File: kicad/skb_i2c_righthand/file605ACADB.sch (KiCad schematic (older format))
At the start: 108 parts, among them SW1 SW_PUSH, SW10 SW_PUSH, SW11 SW_PUSH, SW12 SW_PUSH, SW13 SW_PUSH, SW14 SW_PUSH, SW15 SW_PUSH, SW16 SW_PUSH, SW17 SW_PUSH, SW18 SW_PUSH, SW19 SW_PUSH, SW2 SW_PUSH, SW20 SW_PUSH, SW21 SW_PUSH, SW22 SW_PUSH, SW23 SW_PUSH, SW24 SW_PUSH, SW25 SW_PUSH, SW26 SW_PUSH, SW27 SW_PUSH, SW28 SW_PUSH, SW29 SW_PUSH, SW3 SW_PUSH, SW30 SW_PUSH, SW31 SW_PUSH, SW32 SW_PUSH, SW33 SW_PUSH, SW34 SW_PUSH, SW35 SW_PUSH, SW36 SW_PUSH, SW37 SW_PUSH, SW38 SW_PUSH, SW39 SW_PUSH, SW4 SW_PUSH, SW40 SW_PUSH, SW41 SW_PUSH, SW42 SW_PUSH, SW43 SW_PUSH, SW44 SW_PUSH, SW45 SW_PUSH, SW46 SW_PUSH, SW47 SW_PUSH, SW48 SW_PUSH, SW49 SW_PUSH, SW5 SW_PUSH, SW50 SW_PUSH, SW51 SW_PUSH, SW52 SW_PUSH, SW53 SW_PUSH, SW54 SW_PUSH, SW6 SW_PUSH, SW7 SW_PUSH, SW8 SW_PUSH, SW9 SW_PUSH

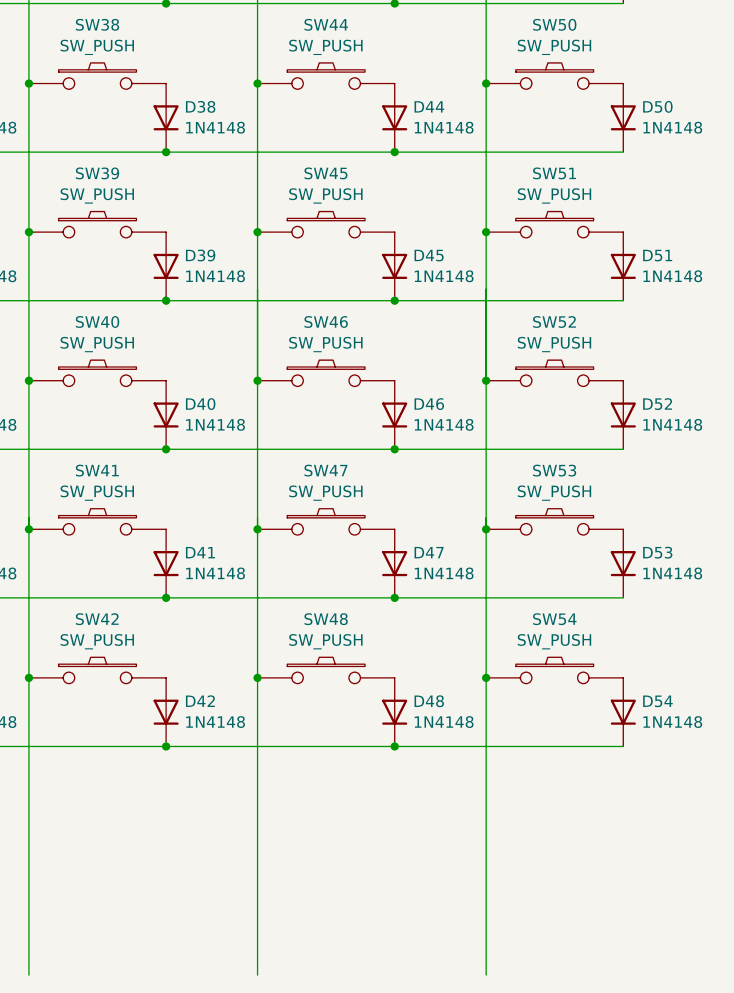
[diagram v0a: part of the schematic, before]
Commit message: route roughly
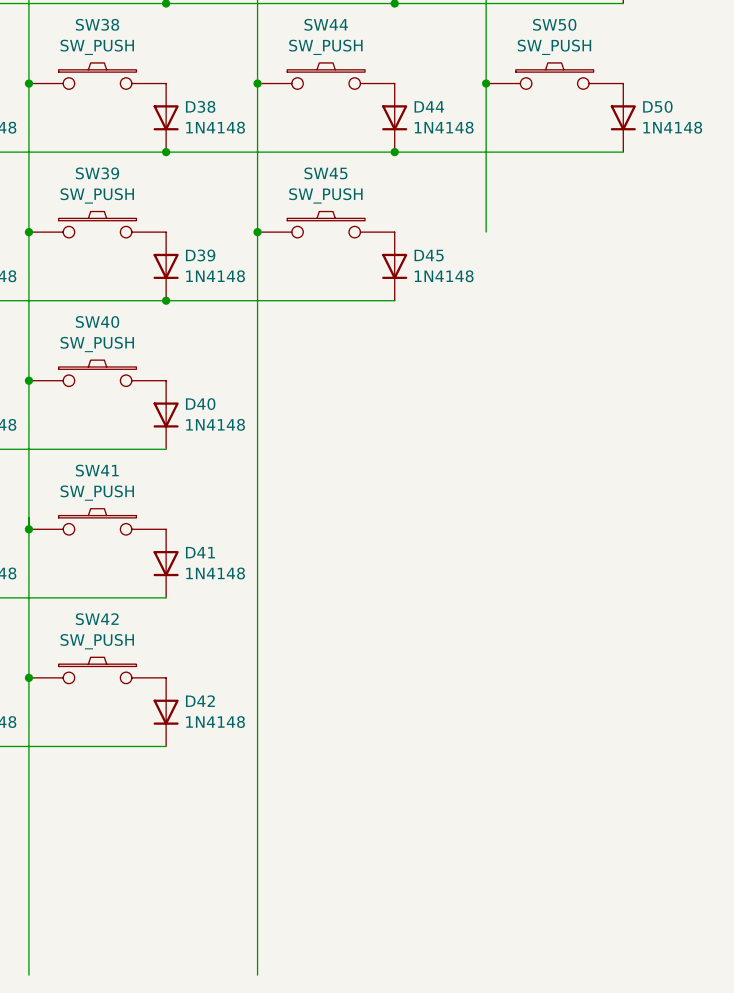
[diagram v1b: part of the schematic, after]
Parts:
- removed D46, D47, D48, D51, D52, D53, D54: 1N4148, Diode_THT:D_DO-35_SOD27_P7.62mm_Horizontal, symbol Diode:1N4148
- removed SW46, SW47, SW48, SW51, SW52, SW53, SW54: SW_PUSH, keyboard_parts:Kailh_MX_Socket, symbol kbd:SW_PUSH
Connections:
- wire segments 129 -> 111
